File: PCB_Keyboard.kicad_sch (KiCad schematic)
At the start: 24 parts, among them SW1 SW_Push, U1 ATmega32U4-A, Y1 16MHz

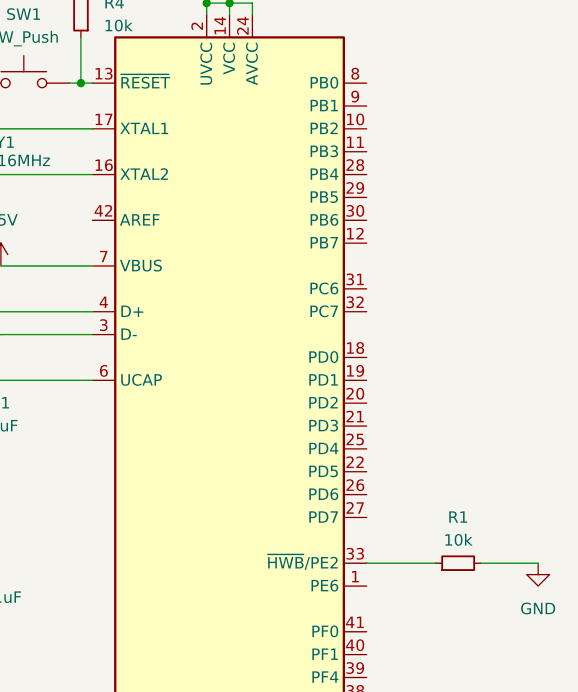
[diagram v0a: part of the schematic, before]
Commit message: roteamento
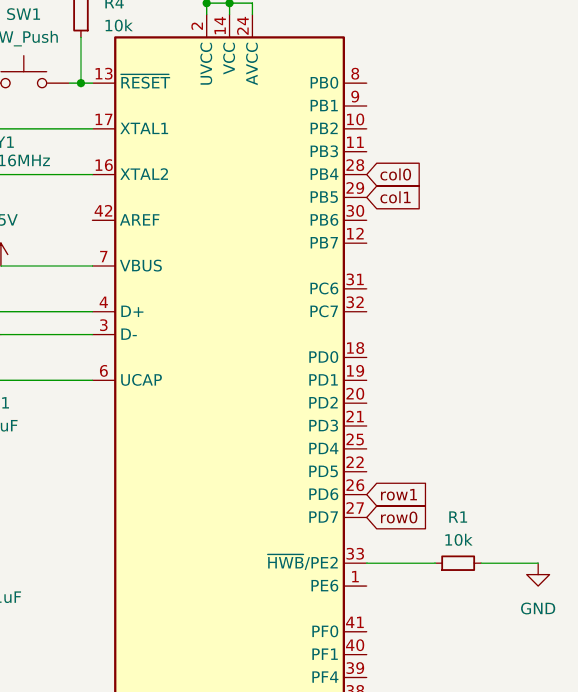
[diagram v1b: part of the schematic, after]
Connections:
- net col0: now also U1.28 (PB4)
- net col1: now also U1.29 (PB5)
- net row0: now also U1.27 (PD7)
- net row1: now also U1.26 (PD6)
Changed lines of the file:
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@@
 	(global_label "col1"
 		(shape input)
+		(at 154.94 69.85 0)
+		(fields_autoplaced yes)
+		(effects
+			(font
+				(size 1.27 1.27)
+			)
+			(justify left)
+		)
+		(property "Intersheetrefs" "${INTERSHEET_REFS}"
+			(at 162.0375 69.85 0)
+			(effects
+				(font
+					(size 1.27 1.27)
+				)
+				(justify left)
+				(hide yes)
+			)
+		)
+	)
+	(global_label "col1"
+		(shape input)
 		(at 58.42 62.23 90)
 		(fields_autoplaced yes)
@@
 	(global_label "col0"
 		(shape input)
+		(at 154.94 67.31 0)
+		(fields_autoplaced yes)
+		(effects
+			(font
+				(size 1.27 1.27)
+			)
+			(justify left)
+		)
+		(property "Intersheetrefs" "${INTERSHEET_REFS}"
+			(at 162.0375 67.31 0)
+			(effects
+				(font
+					(size 1.27 1.27)
+				)
+				(justify left)
+				(hide yes)
+			)
+		)
+	)
+	(global_label "col0"
+		(shape input)
 		(at 41.91 62.23 90)
 		(fields_autoplaced yes)
@@
 			(effects
 				(font
+					(size 1.27 1.27)
+				)
+				(justify left)
+				(hide yes)
+			)
+		)
+	)
+	(global_label "row1"
+		(shape input)
+		(at 154.94 102.87 0)
+		(fields_autoplaced yes)
+		(effects
+			(font
+				(size 1.27 1.27)
+			)
+			(justify left)
+		)
+		(property "Intersheetrefs" "${INTERSHEET_REFS}"
+			(at 162.4004 102.87 0)
+			(effects
+				(font
+					(size 1.27 1.27)
+				)
+				(justify left)
+				(hide yes)
+			)
+		)
+	)
+	(global_label "row0"
+		(shape input)
+		(at 154.94 105.41 0)
+		(fields_autoplaced yes)
+		(effects
+			(font
+				(size 1.27 1.27)
+			)
+			(justify left)
+		)
+		(property "Intersheetrefs" "${INTERSHEET_REFS}"
+			(at 162.4004 105.41 0)
+			(effects
+				(font
